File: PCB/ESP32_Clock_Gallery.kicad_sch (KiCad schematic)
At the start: 0 parts

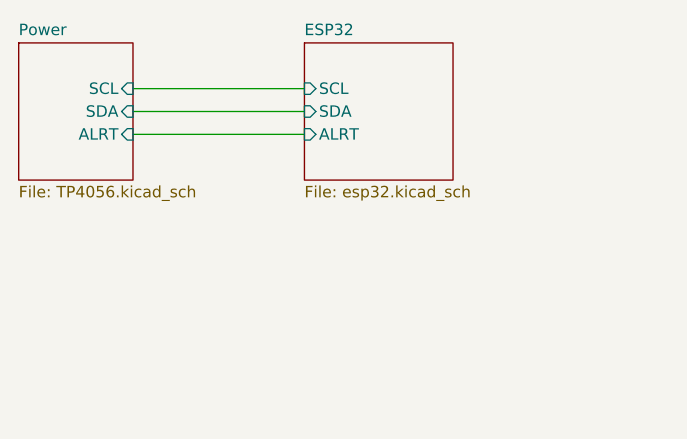
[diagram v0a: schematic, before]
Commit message: PCB Routing
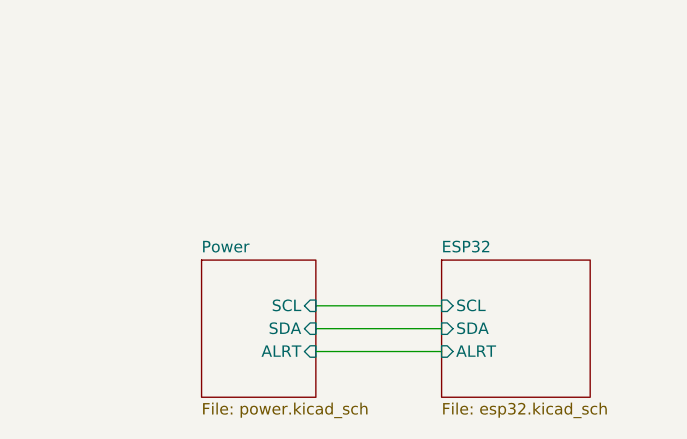
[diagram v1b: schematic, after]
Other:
- sheet Power: file TP4056.kicad_sch -> power.kicad_sch
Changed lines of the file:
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@@
 	(wire
 		(pts
-			(xy 106.68 78.74) (xy 125.73 78.74)
+			(xy 127 102.87) (xy 140.97 102.87)
 		)
 		(stroke
@@
 	(wire
 		(pts
-			(xy 106.68 76.2) (xy 125.73 76.2)
+			(xy 127 100.33) (xy 140.97 100.33)
 		)
 		(stroke
@@
 	(wire
 		(pts
-			(xy 106.68 73.66) (xy 125.73 73.66)
+			(xy 127 97.79) (xy 140.97 97.79)
 		)
 		(stroke
@@
 	)
 	(sheet
-		(at 125.73 68.58)
+		(at 140.97 92.71)
 		(size 16.51 15.24)
 		(fields_autoplaced yes)
@@
 		)
 		(property "Sheetname" "ESP32"
-			(at 125.73 67.8684 0)
+			(at 140.97 91.9984 0)
 			(effects
 				(font
@@
 		)
 		(property "Sheetfile" "esp32.kicad_sch"
-			(at 125.73 84.4046 0)
+			(at 140.97 108.5346 0)
 			(effects
 				(font
@@
 		)
 		(pin "SCL" input
-			(at 125.73 73.66 180)
+			(at 140.97 97.79 180)
 			(effects
 				(font
@@
 		)
 		(pin "SDA" input
-			(at 125.73 76.2 180)
+			(at 140.97 100.33 180)
 			(effects
 				(font
@@
 		)
 		(pin "ALRT" input
-			(at 125.73 78.74 180)
+			(at 140.97 102.87 180)
 			(effects
 				(font
@@
 	)
 	(sheet
-		(at 93.98 68.58)
+		(at 114.3 92.71)
 		(size 12.7 15.24)
 		(fields_autoplaced yes)
@@
 		)
 		(property "Sheetname" "Power"
-			(at 93.98 67.8684 0)
+			(at 114.3 91.9984 0)
 			(effects
 				(font
@@
 			)
 		)
-		(property "Sheetfile" "TP4056.kicad_sch"
-			(at 93.98 84.4046 0)
+		(property "Sheetfile" "power.kicad_sch"
+			(at 114.3 108.5346 0)
 			(effects
 				(font
@@
 		)
 		(pin "SCL" input
-			(at 106.68 73.66 0)
+			(at 127 97.79 0)
 			(effects
 				(font
@@
 		)
 		(pin "SDA" input
-			(at 106.68 76.2 0)
+			(at 127 100.33 0)
 			(effects
 				(font
@@
 		)
 		(pin "ALRT" input
-			(at 106.68 78.74 0)
+			(at 127 102.87 0)
 			(effects
 				(font
